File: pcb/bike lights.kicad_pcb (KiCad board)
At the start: 2 copper layers, 122.2 x 104.8 mm, 47 parts, among them SW1 JST_EH_B2B-EH-A_1x02_P2.50mm_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, SW2 JST_EH_B3B-EH-A_1x03_P2.50mm_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

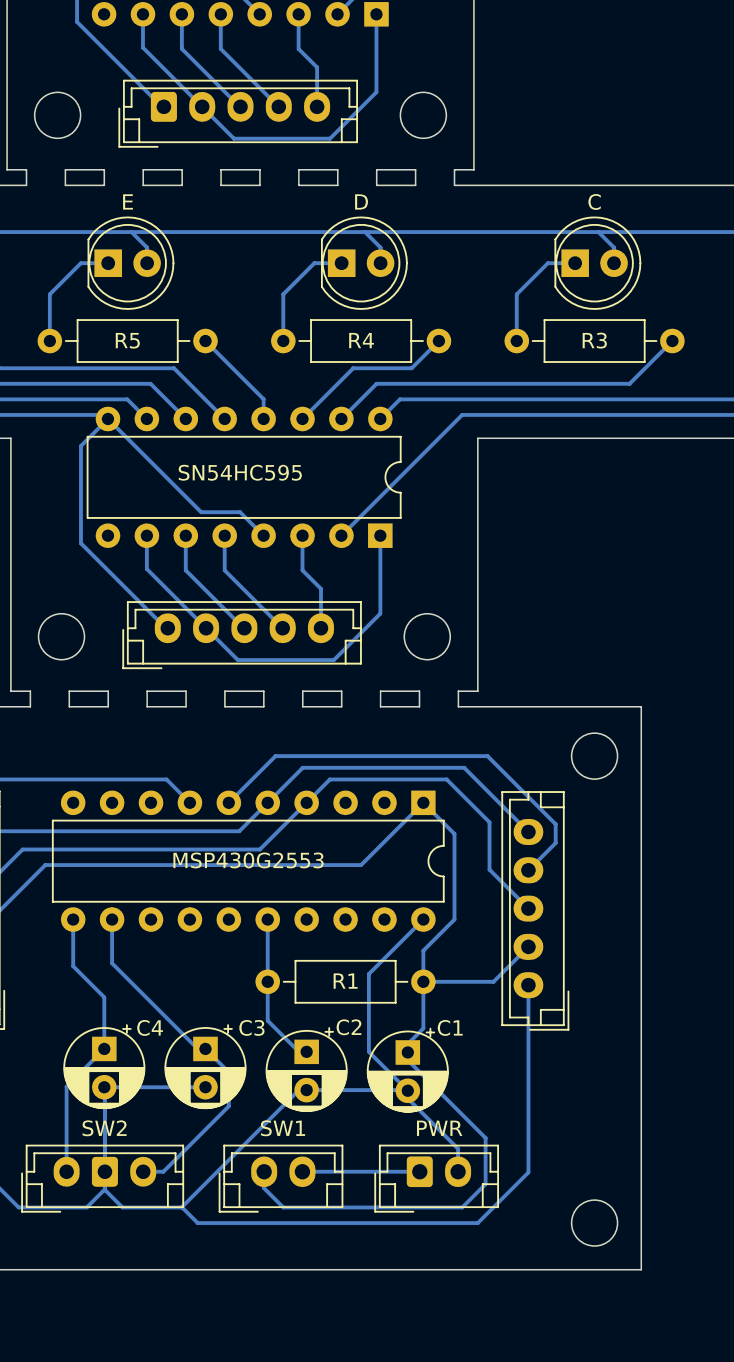
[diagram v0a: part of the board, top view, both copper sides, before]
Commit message: Update pcb design
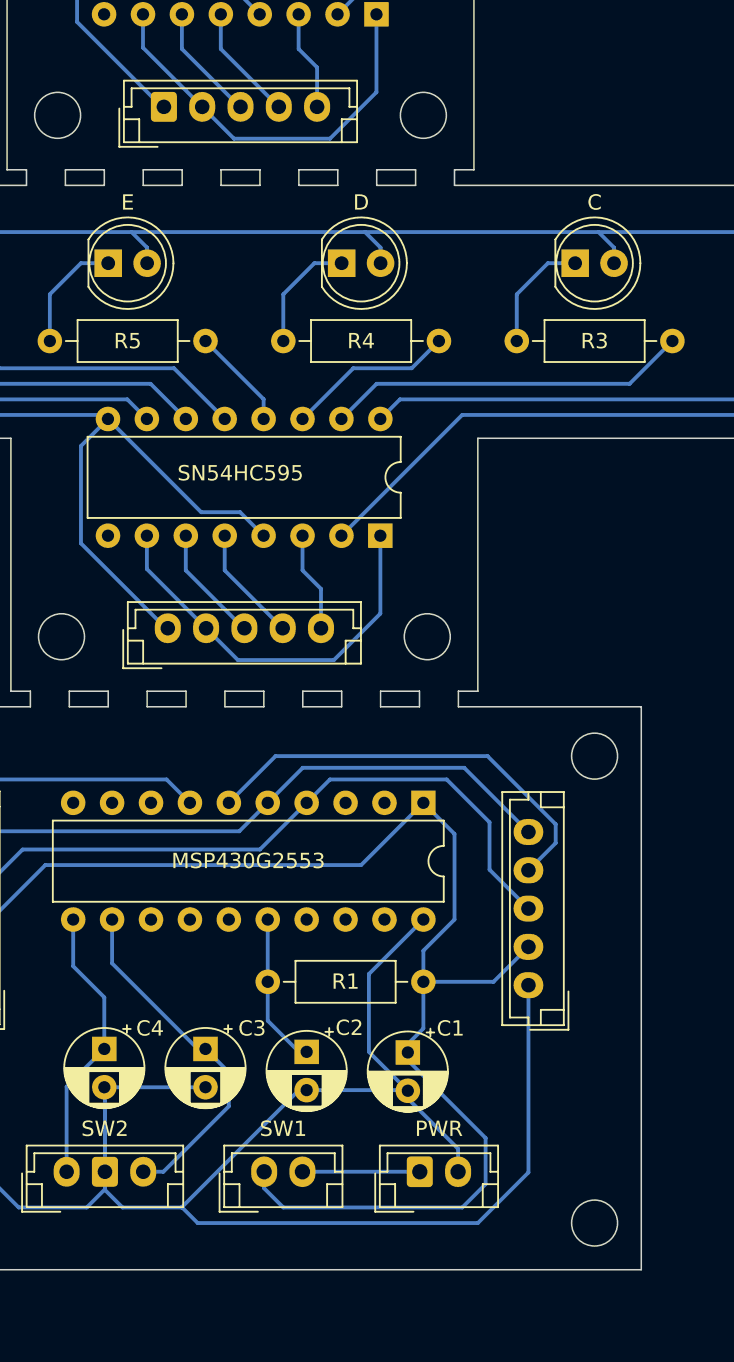
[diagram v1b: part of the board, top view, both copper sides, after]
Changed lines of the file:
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@@
       (outputformat 1)
       (mirror false)
-      (drillshape 1)
+      (drillshape 0)
       (scaleselection 1)
-      (outputdirectory "")
+      (outputdirectory "gbr/")
     )
   )
@@
     (pad "1" thru_hole oval (at 0 0) (size 1.7 1.95) (drill 0.95) (layers "*.Cu" "*.Mask")
       (net 10 "SWITCH_1"))
-    (pad "2" thru_hole roundrect (at 2.5 0) (size 1.7 1.95) (drill 0.95) (layers "*.Cu" "*.Mask") (roundrect_rratio 0.147059)
+    (pad "2" thru_hole roundrect (at 2.5 0) (size 1.7 1.95) (drill 0.95) (layers "*.Cu" "*.Mask") (roundrect_rratio 0.1470588235)
       (net 2 "GND"))
     (pad "3" thru_hole oval (at 5 0) (size 1.7 1.95) (drill 0.95) (layers "*.Cu" "*.Mask")
@@
     (fp_line (start 5 2.2) (end 5 -1.6)
       (stroke (width 0.1) (type solid)) (layer "F.Fab"))
-    (pad "1" thru_hole roundrect (at 0 0) (size 1.7 2) (drill 1) (layers "*.Cu" "*.Mask") (roundrect_rratio 0.147059)
+    (pad "1" thru_hole roundrect (at 0 0) (size 1.7 2) (drill 1) (layers "*.Cu" "*.Mask") (roundrect_rratio 0.1470588235)
       (net 1 "VCC"))
     (pad "2" thru_hole oval (at 2.5 0) (size 1.7 2) (drill 1) (layers "*.Cu" "*.Mask")
@@
     (fp_line (start 12.5 2.2) (end 12.5 -1.6)
       (stroke (width 0.1) (type solid)) (layer "F.Fab"))
-    (pad "1" thru_hole roundrect (at 0 0) (size 1.7 1.95) (drill 0.95) (layers "*.Cu" "*.Mask") (roundrect_rratio 0.147059)
+    (pad "1" thru_hole roundrect (at 0 0) (size 1.7 1.95) (drill 0.95) (layers "*.Cu" "*.Mask") (roundrect_rratio 0.1470588235)
       (net 2 "GND"))
     (pad "2" thru_hole oval (at 2.5 0) (size 1.7 1.95) (drill 0.95) (layers "*.Cu" "*.Mask")
@@
   (gr_circle (center 125.984 129.714) (end 127.484 129.714)
     (stroke (width 0.1) (type default)) (fill none) (layer "Edge.Cuts"))
+  (gr_line (start 174.752 163.242) (end 174.752 126.492)
+    (stroke (width 0.1) (type default)) (layer "Edge.Cuts"))
   (gr_line (start 142.494 125.476) (end 145.034 125.476)
     (stroke (width 0.1) (type default)) (layer "Edge.Cuts"))
@@
   (gr_line (start 87.884 92.456) (end 134.62 92.456)
     (stroke (width 0.1) (type default)) (layer "Edge.Cuts"))
-  (gr_line (start 174.752 163.2458) (end 174.752 126.492)
-    (stroke (width 0.1) (type default)) (layer "Edge.Cuts"))
   (gr_line (start 145.034 126.492) (end 145.034 125.476)
